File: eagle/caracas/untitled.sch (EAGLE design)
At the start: 24 parts, among them IC1 4001N, Q1 IRLZ44Z, X1 22-23-2021, X2 22-23-2021, X3 22-23-2021, X4 22-23-2041, X5 22-23-2021, X6 22-23-2041

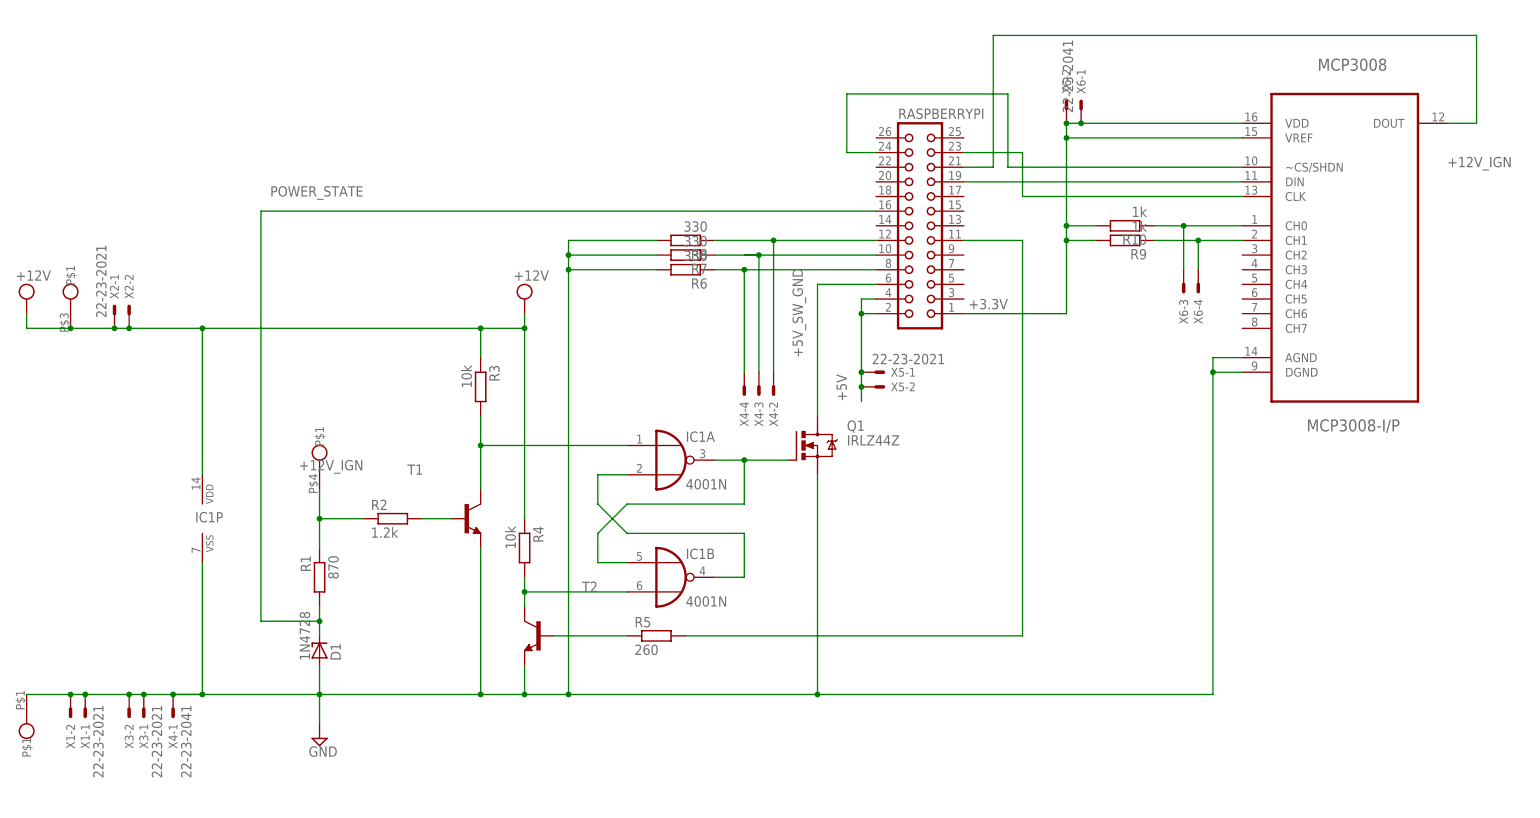
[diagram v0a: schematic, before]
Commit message: Possibly last version of schematics.
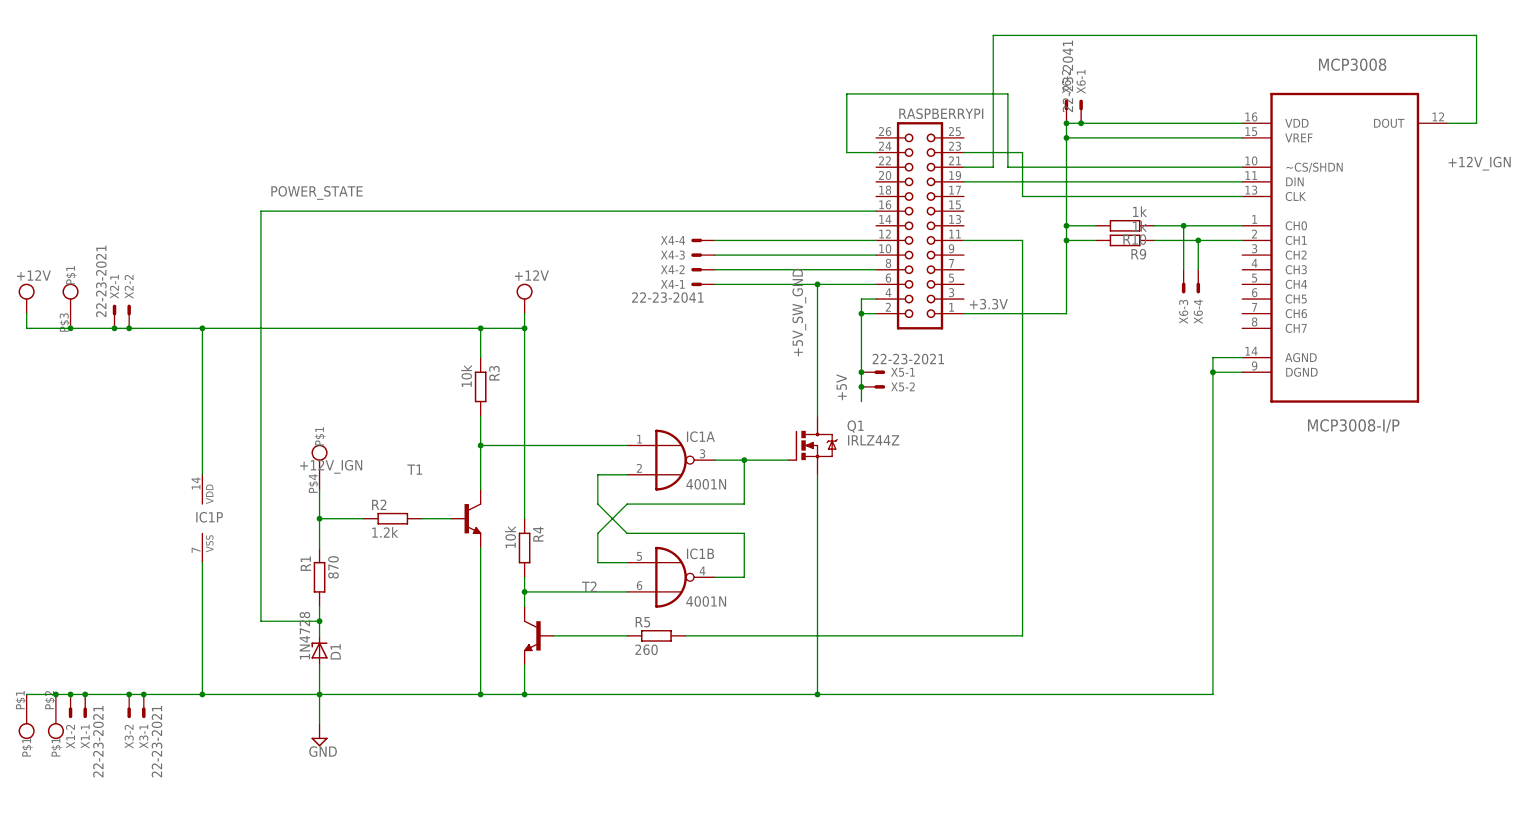
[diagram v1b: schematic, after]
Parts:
- removed R6, R7, R8: 330, rcl:R-EU_0207/10
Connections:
- net +5V_SW_GND: now also X4-1.S
- net GND: now also U$1G$2.P$1; no longer R6.2, R7.2, R8.2, X4-1.S
- net N$10: now also X4-4.S; no longer R8.1, X4-2.S
- net N$7: now also X4-2.S; no longer R6.1, X4-4.S
- net N$8: no longer R7.1
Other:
- moved on the sheet: X4-1, X4-2, X4-3, X4-4
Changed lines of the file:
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@@
 <class number="0" name="default" width="0" drill="0">
 </class>
-<class number="1" name="Ground" width="0.6096" drill="0">
+<class number="1" name="Ground" width="0.4064" drill="0">
 <clearance class="1" value="0.3048"/>
 </class>
@@
 <part name="R10" library="rcl" deviceset="R-EU_" device="0207/10" value="1k"/>
 <part name="R9" library="rcl" deviceset="R-EU_" device="0207/10" value="1k"/>
-<part name="R6" library="rcl" deviceset="R-EU_" device="0207/10" value="330"/>
-<part name="R7" library="rcl" deviceset="R-EU_" device="0207/10" value="330"/>
-<part name="R8" library="rcl" deviceset="R-EU_" device="0207/10" value="330"/>
 <part name="X2" library="con-molex" deviceset="22-23-2021" device=""/>
 <part name="X3" library="con-molex" deviceset="22-23-2021" device=""/>
@@
 <instance part="R10" gate="G$1" x="-38.1" y="27.94" rot="R180"/>
 <instance part="R9" gate="G$1" x="-38.1" y="25.4" rot="R180"/>
-<instance part="R6" gate="G$1" x="-114.3" y="20.32" rot="R180"/>
-<instance part="R7" gate="G$1" x="-114.3" y="22.86" rot="R180"/>
-<instance part="R8" gate="G$1" x="-114.3" y="25.4" rot="R180"/>
 <instance part="X2" gate="-1" x="-213.36" y="12.7" rot="R90"/>
 <instance part="X2" gate="-2" x="-210.82" y="12.7" rot="R90"/>
@@
 <instance part="X1" gate="-2" x="-220.98" y="-55.88" rot="R270"/>
 <instance part="X6" gate="-1" x="-45.72" y="48.26" rot="R90"/>
-<instance part="X4" gate="-2" x="-99.06" y="0" rot="R270"/>
-<instance part="X4" gate="-3" x="-101.6" y="0" rot="R270"/>
-<instance part="X4" gate="-4" x="-104.14" y="0" rot="R270"/>
-<instance part="X4" gate="-1" x="-203.2" y="-55.88" rot="R270"/>
+<instance part="X4" gate="-2" x="-111.76" y="20.32" rot="R180"/>
+<instance part="X4" gate="-3" x="-111.76" y="22.86" rot="R180"/>
+<instance part="X4" gate="-4" x="-111.76" y="25.4" rot="R180"/>
 <instance part="X6" gate="-4" x="-25.4" y="17.78" rot="R270"/>
 <instance part="X6" gate="-3" x="-27.94" y="17.78" rot="R270"/>
@@
 <instance part="T1" gate="G$1" x="-152.4" y="-22.86"/>
 <instance part="R2" gate="G$1" x="-165.1" y="-22.86"/>
+<instance part="X4" gate="-1" x="-111.76" y="17.78" rot="R180"/>
+<instance part="U$1" gate="G$2" x="-223.52" y="-58.42" rot="R270"/>
 </instances>
 <busses>
@@
 <segment>
 <pinref part="U$1" gate="G$1" pin="P$1"/>
-<wire x1="-228.6" y1="-53.34" x2="-220.98" y2="-53.34" width="0.1524" layer="91"/>
+<wire x1="-228.6" y1="-53.34" x2="-223.52" y2="-53.34" width="0.1524" layer="91"/>
 <pinref part="X3" gate="-1" pin="S"/>
+<wire x1="-223.52" y1="-53.34" x2="-220.98" y2="-53.34" width="0.1524" layer="91"/>
 <wire x1="-220.98" y1="-53.34" x2="-218.44" y2="-53.34" width="0.1524" layer="91"/>
 <wire x1="-218.44" y1="-53.34" x2="-210.82" y2="-53.34" width="0.1524" layer="91"/>
 <wire x1="-210.82" y1="-53.34" x2="-208.28" y2="-53.34" width="0.1524" layer="91"/>
-<wire x1="-208.28" y1="-53.34" x2="-203.2" y2="-53.34" width="0.1524" layer="91"/>
 <junction x="-208.28" y="-53.34"/>
 <pinref part="X3" gate="-2" pin="S"/>
@@
 <junction x="-220.98" y="-53.34"/>
 <pinref part="IC1" gate="P" pin="VSS"/>
-<wire x1="-198.12" y1="-53.34" x2="-203.2" y2="-53.34" width="0.1524" layer="91"/>
+<wire x1="-198.12" y1="-53.34" x2="-208.28" y2="-53.34" width="0.1524" layer="91"/>
 <wire x1="-198.12" y1="-30.48" x2="-198.12" y2="-53.34" width="0.1524" layer="91"/>
 <junction x="-198.12" y="-53.34"/>
-<pinref part="X4" gate="-1" pin="S"/>
-<junction x="-203.2" y="-53.34"/>
 <pinref part="SUPPLY2" gate="GND" pin="GND"/>
 <pinref part="D1" gate="1" pin="A"/>
@@
 <pinref part="Q1" gate="G$1" pin="S"/>
 <wire x1="-91.44" y1="-15.24" x2="-91.44" y2="-53.34" width="0.1524" layer="91"/>
-<wire x1="-91.44" y1="-53.34" x2="-134.62" y2="-53.34" width="0.1524" layer="91"/>
+<wire x1="-91.44" y1="-53.34" x2="-142.24" y2="-53.34" width="0.1524" layer="91"/>
 <junction x="-142.24" y="-53.34"/>
 <pinref part="T1" gate="G$1" pin="E"/>
-<wire x1="-134.62" y1="-53.34" x2="-142.24" y2="-53.34" width="0.1524" layer="91"/>
 <wire x1="-149.86" y1="-27.94" x2="-149.86" y2="-53.34" width="0.1524" layer="91"/>
 <junction x="-149.86" y="-53.34"/>
-<wire x1="-203.2" y1="-53.34" x2="-177.8" y2="-53.34" width="0.1524" layer="91"/>
+<wire x1="-198.12" y1="-53.34" x2="-177.8" y2="-53.34" width="0.1524" layer="91"/>
 <pinref part="MCP3008" gate="A" pin="DGND"/>
 <wire x1="-17.78" y1="2.54" x2="-22.86" y2="2.54" width="0.1524" layer="91"/>
@@
 <wire x1="-22.86" y1="-53.34" x2="-91.44" y2="-53.34" width="0.1524" layer="91"/>
 <junction x="-91.44" y="-53.34"/>
-<pinref part="R8" gate="G$1" pin="2"/>
-<wire x1="-119.38" y1="25.4" x2="-134.62" y2="25.4" width="0.1524" layer="91"/>
-<pinref part="R6" gate="G$1" pin="2"/>
-<wire x1="-119.38" y1="20.32" x2="-134.62" y2="20.32" width="0.1524" layer="91"/>
-<wire x1="-134.62" y1="20.32" x2="-134.62" y2="22.86" width="0.1524" layer="91"/>
-<wire x1="-134.62" y1="22.86" x2="-134.62" y2="25.4" width="0.1524" layer="91"/>
-<pinref part="R7" gate="G$1" pin="2"/>
-<wire x1="-119.38" y1="22.86" x2="-134.62" y2="22.86" width="0.1524" layer="91"/>
-<junction x="-134.62" y="22.86"/>
-<junction x="-134.62" y="20.32"/>
-<wire x1="-134.62" y1="20.32" x2="-134.62" y2="-53.34" width="0.1524" layer="91"/>
-<junction x="-134.62" y="-53.34"/>
+<pinref part="U$1" gate="G$2" pin="P$1"/>
+<junction x="-223.52" y="-53.34"/>
 </segment>
 </net>
@@
 <pinref part="Q1" gate="G$1" pin="D"/>
 <wire x1="-91.44" y1="17.78" x2="-91.44" y2="-5.08" width="0.1524" layer="91"/>
+<pinref part="X4" gate="-1" pin="S"/>
+<wire x1="-109.22" y1="17.78" x2="-91.44" y2="17.78" width="0.1524" layer="91"/>
+<junction x="-91.44" y="17.78"/>
 </segment>
 </net>
@@
 <segment>
 <pinref part="RASPBERRYPI" gate="A" pin="8"/>
-<wire x1="-81.28" y1="20.32" x2="-104.14" y2="20.32" width="0.1524" layer="91"/>
-<wire x1="-104.14" y1="20.32" x2="-109.22" y2="20.32" width="0.1524" layer="91"/>
-<wire x1="-104.14" y1="20.32" x2="-104.14" y2="2.54" width="0.1524" layer="91"/>
-<junction x="-104.14" y="20.32"/>
-<pinref part="R6" gate="G$1" pin="1"/>
+<wire x1="-81.28" y1="20.32" x2="-109.22" y2="20.32" width="0.1524" layer="91"/>
+<pinref part="X4" gate="-2" pin="S"/>
+</segment>
+</net>
+<net name="N$8" class="0">
+<segment>
+<pinref part="RASPBERRYPI" gate="A" pin="10"/>
+<wire x1="-81.28" y1="22.86" x2="-109.22" y2="22.86" width="0.1524" layer="91"/>
+<pinref part="X4" gate="-3" pin="S"/>
+</segment>
+</net>
+<net name="N$10" class="0">
+<segment>
+<pinref part="RASPBERRYPI" gate="A" pin="12"/>
+<wire x1="-81.28" y1="25.4" x2="-109.22" y2="25.4" width="0.1524" layer="91"/>
 <pinref part="X4" gate="-4" pin="S"/>
 </segment>
 </net>
-<net name="N$8" class="0">
-<segment>
-<pinref part="RASPBERRYPI" gate="A" pin="10"/>
-<wire x1="-81.28" y1="22.86" x2="-101.6" y2="22.86" width="0.1524" layer="91"/>
-<wire x1="-104.14" y1="22.86" x2="-101.6" y2="22.86" width="0.1524" layer="91"/>
-<wire x1="-101.6" y1="22.86" x2="-109.22" y2="22.86" width="0.1524" layer="91"/>
-<wire x1="-101.6" y1="22.86" x2="-101.6" y2="2.54" width="0.1524" layer="91"/>
-<junction x="-101.6" y="22.86"/>
-<pinref part="R7" gate="G$1" pin="1"/>
-<pinref part="X4" gate="-3" pin="S"/>
-</segment>
-</net>
-<net name="N$10" class="0">
-<segment>
-<pinref part="RASPBERRYPI" gate="A" pin="12"/>
-<wire x1="-81.28" y1="25.4" x2="-99.06" y2="25.4" width="0.1524" layer="91"/>
-<wire x1="-99.06" y1="25.4" x2="-109.22" y2="25.4" width="0.1524" layer="91"/>
-<wire x1="-99.06" y1="2.54" x2="-99.06" y2="25.4" width="0.1524" layer="91"/>
-<junction x="-99.06" y="25.4"/>
-<pinref part="R8" gate="G$1" pin="1"/>
-<pinref part="X4" gate="-2" pin="S"/>
-</segment>
-</net>
